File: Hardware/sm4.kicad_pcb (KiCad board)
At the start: 4 copper layers, 60 x 55 mm, 93 parts, among them J1 Motor1, J2 Termination, J3 CAN bus, J4 Motor2, J5 I2C, J6 Power, J7 USB_C_Receptacle_USB2.0, J8 Conn_01x05_Male, Q1 NDT2955, SW1 RST_SW, SW2 BOOT_SW, U1 STM32F405RGTx, U2 TMC2100-TA, U3 MCP2562-E-SN, U4 TMC2100-TA, U6 MCP1700-3302E_SOT23, U7 USBLC6-2SC6, Y1 25 MHz

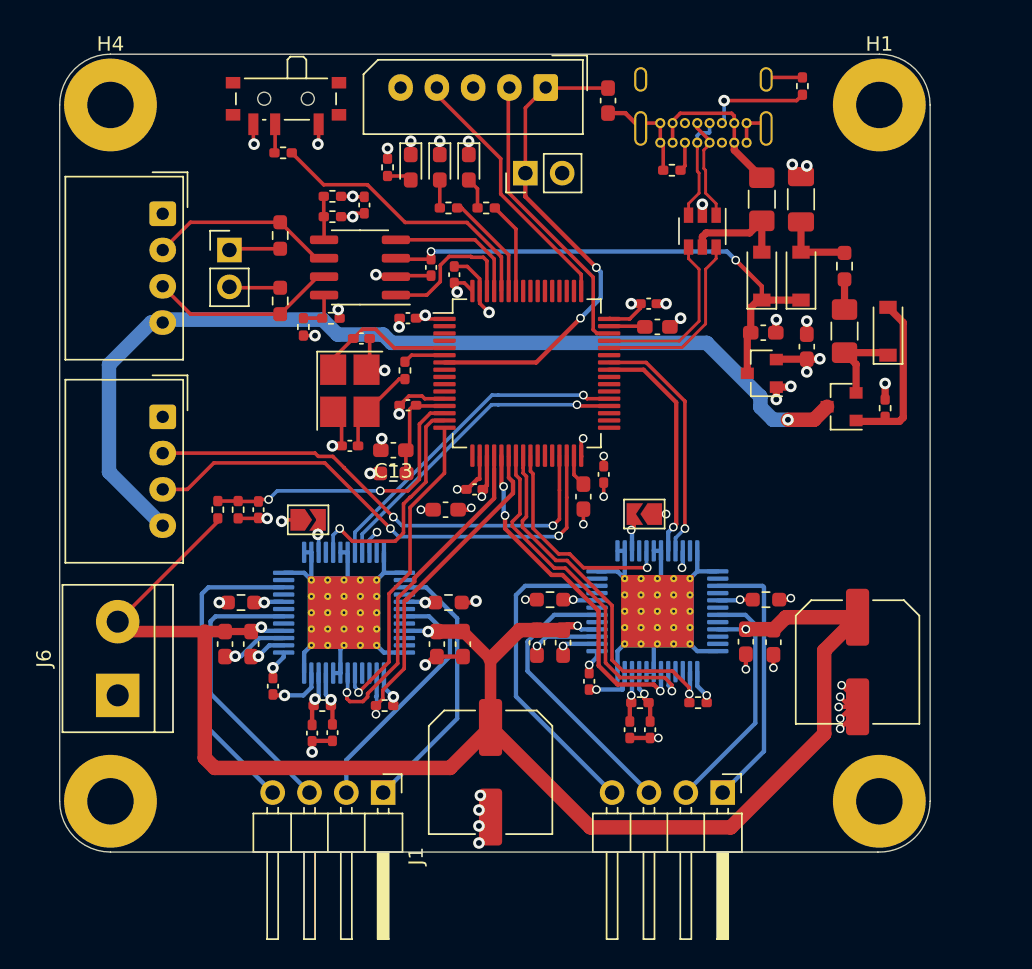
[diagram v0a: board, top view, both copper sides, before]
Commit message: Finalize first HW version. Update firmware project.
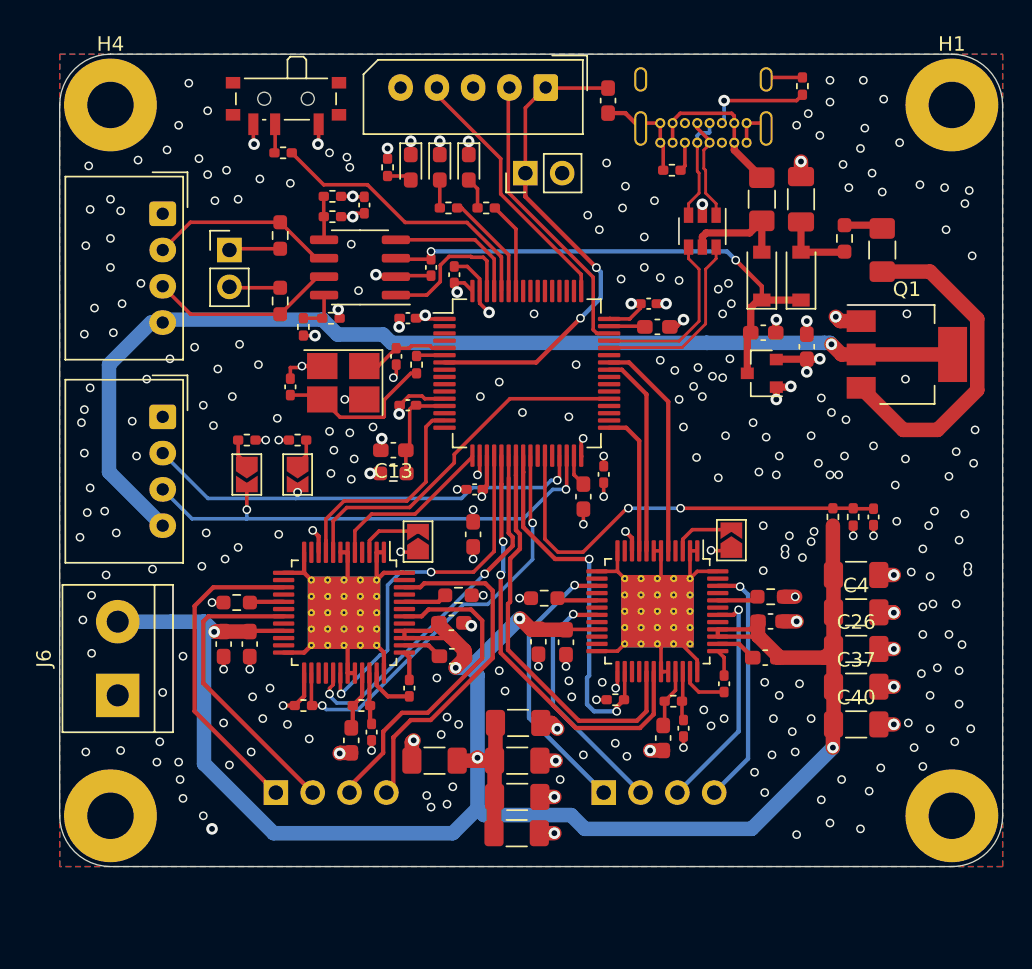
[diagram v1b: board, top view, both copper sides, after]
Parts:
- removed D1: 4V7, Diode_SMD:D_SOD-123
- removed R9: 10k, Resistor_SMD:R_0402_1005Metric_Pad0.72x0.64mm_HandSolder
- added C27: 10u, Capacitor_SMD:C_1206_3216Metric_Pad1.33x1.80mm_HandSolder, F.Cu at (94.9, 85.9)
- added C37: 10u, Capacitor_SMD:C_1206_3216Metric_Pad1.33x1.80mm_HandSolder, F.Cu at (94.9, 93.6)
- added C38: 10u, Capacitor_SMD:C_1206_3216Metric_Pad1.33x1.80mm_HandSolder, F.Cu at (71.5, 103.7)
- added C39: 10u, Capacitor_SMD:C_1206_3216Metric_Pad1.33x1.80mm_HandSolder, F.Cu at (71.6, 96.1)
- added C40: 10u, Capacitor_SMD:C_1206_3216Metric_Pad1.33x1.80mm_HandSolder, F.Cu at (94.9, 96.2)
- added C41: 10u, Capacitor_SMD:C_1206_3216Metric_Pad1.33x1.80mm_HandSolder, F.Cu at (65.8, 98.7)
- added C42: 10u, Capacitor_SMD:C_1206_3216Metric_Pad1.33x1.80mm_HandSolder, F.Cu at (71.5, 98.7)
- added C43: 10u, Capacitor_SMD:C_1206_3216Metric_Pad1.33x1.80mm_HandSolder, F.Cu at (71.5, 101.2)
- added JP3: Jumper_2_Open, Jumper:SolderJumper-2_P1.3mm_Open_TrianglePad1.0x1.5mm, F.Cu at (52.9, 79.0)
- added JP4: Jumper_2_Open, Jumper:SolderJumper-2_P1.3mm_Open_TrianglePad1.0x1.5mm, F.Cu at (56.4, 79.0)
- added R25: 2k2, Resistor_SMD:R_0402_1005Metric_Pad0.72x0.64mm_HandSolder, F.Cu at (52.9, 76.6)
- added R26: 2k2, Resistor_SMD:R_0402_1005Metric_Pad0.72x0.64mm_HandSolder, F.Cu at (56.4, 76.6)
- C26, C4: value 47u -> 10u; footprint Capacitor_SMD:C_Elec_8x6.2 -> Capacitor_SMD:C_1206_3216Metric_Pad1.33x1.80mm_HandSolder
- C30, C7: value 470n -> 4u7; footprint Capacitor_SMD:C_0402_1005Metric_Pad0.74x0.62mm_HandSolder -> Capacitor_SMD:C_0603_1608Metric_Pad1.08x0.95mm_HandSolder
- J1, J4: moved to B.Cu
- Q1: footprint Package_TO_SOT_SMD:SOT-23 -> Package_TO_SOT_SMD:SOT-223-3_TabPin2
- U2, U4: moved to F.Cu
- moved R19 42.4 mm to (94.7, 81.9)
- moved R18 42.4 mm to (93.3, 81.9)
- moved C36 42.4 mm to (96.1, 81.9)
- moved C26 26.6 mm to (94.9, 91.0), turned to 0 degrees
- moved C24 16.2 mm to (89.0, 89.1), turned to 0 degrees
- moved C3 15.7 mm to (67.0, 89.2), turned to 0 degrees
- moved R16 15.3 mm to (73.4, 87.5), turned to 0 degrees
- moved R17 15.2 mm to (89.0, 87.4), turned to 180 degrees
- moved R5 15.0 mm to (67.5, 87.3), turned to 180 degrees
- moved C6 14.7 mm to (51.3, 90.7)
- moved C5 14.7 mm to (53.1, 90.7)
- moved R3 14.6 mm to (52.2, 87.8), turned to 0 degrees
- moved C28 14.3 mm to (73.0, 90.5)
- moved C29 14.3 mm to (74.9, 90.5)
- moved C23 14.0 mm to (88.6, 91.6), turned to 180 degrees
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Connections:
- C24 pad 2: VSA2 -> GND
- C3 pad 2: VSA1 -> GND
- F1 pad 2: Net-(D1-Pad1) -> Net-(F1-Pad2)
- Q1 pad 1: Net-(D1-Pad2) -> GND
- Q1 pad 2: Net-(D1-Pad1) -> VDC
- Q1 pad 3: VDC -> Net-(F1-Pad2)
- U1 pad 14: VBAT -> (no net)
- U1 pad 15: MODE1 -> DIR1
- U1 pad 16: EN1 -> (no net)
- U1 pad 17: (no net) -> MODE1
- U1 pad 22: ERR1 -> EN1
- U1 pad 25: MODE2 -> ERR1
- U1 pad 27: (no net) -> VBAT
- U1 pad 33: (no net) -> DIR2
- U1 pad 36: DIR1 -> (no net)
- U1 pad 42: DIR2 -> MODE2
- U2 pad 39: VSA1 -> VS1
- U4 pad 39: VSA2 -> VS1
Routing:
- net VS1: track 119.5 -> 143.5 mm, vias 4 -> 5
- net Net-(F1-Pad2): track 0.00 -> 23.2 mm
- net Net-(D1-Pad2): track 11.4 -> 0.00 mm
- net VBAT: track 20.4 -> 30.0 mm
- net DIR2: track 16.9 -> 10.0 mm, vias 1 -> 0
- net DIR1: track 22.0 -> 15.5 mm, vias 1 -> 0
- net Net-(D1-Pad1): track 6.18 -> 0.00 mm
- net VDC: track 67.1 -> 73.1 mm
- net REF2: track 24.0 -> 29.8 mm, vias 3 -> 2
- net Net-(J4-Pad4): track 22.2 -> 17.0 mm, vias 0 -> 1
- net Net-(C17-Pad1): track 6.17 -> 11.2 mm
- net VSA2: track 5.03 -> 0.00 mm, vias 1 -> 0
- net VSA1: track 4.57 -> 0.00 mm, vias 1 -> 0
- net MODE1: track 16.3 -> 11.8 mm, vias 1 -> 0
- net GND: track 153.9 -> 149.5 mm, vias 46 -> 286
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- added copper zone on B.Cu, net GND
- added copper zone on F.Cu, net GND
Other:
- board size 60 x 55 mm -> 65 x 56 mm
